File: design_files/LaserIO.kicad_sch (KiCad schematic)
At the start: 25 parts, among them J10 DA15_Receptacle, J11 DB25_Receptacle, U4 74HC245, U5 UA9638CDR, U6 UA9638CDR, U7 74LVC1G3208

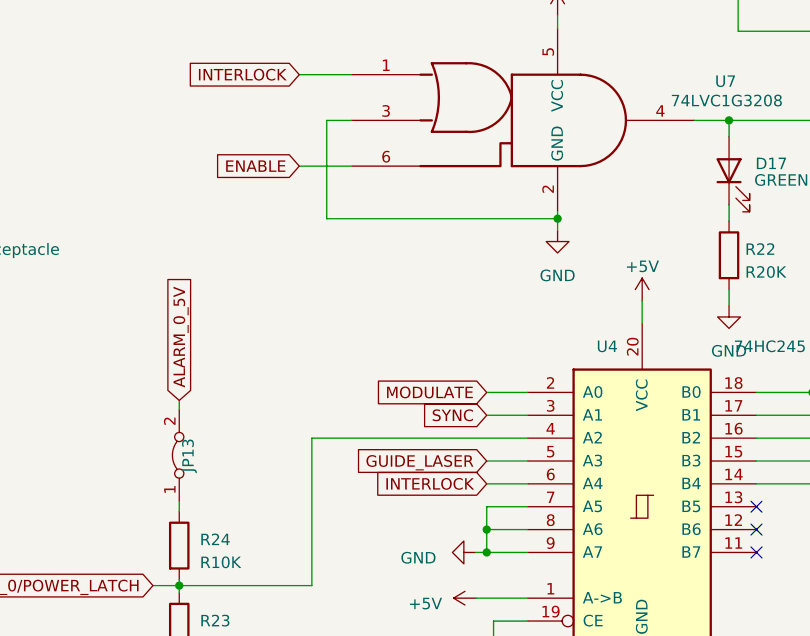
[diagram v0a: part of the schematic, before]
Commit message: Rev 5a
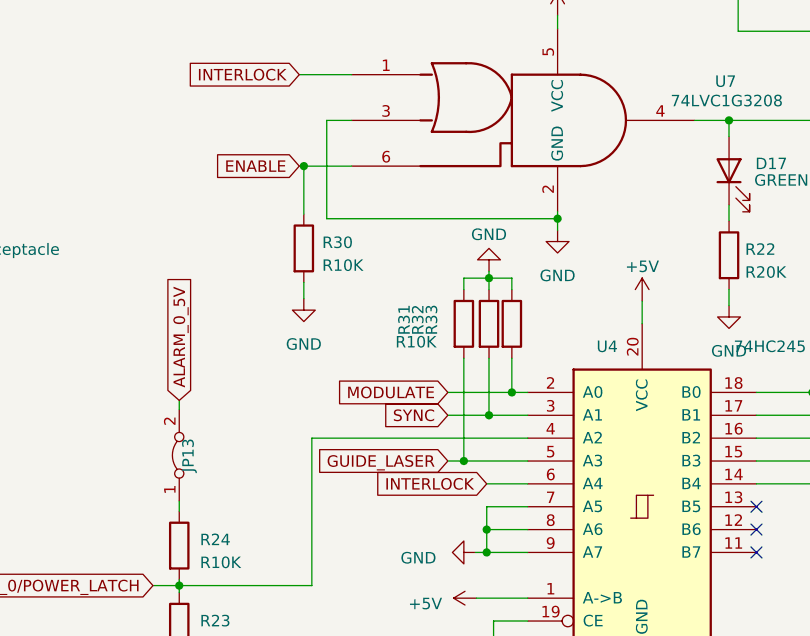
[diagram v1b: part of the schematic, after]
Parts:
- added R30, R31, R32, R33: R10K, LaserBoardR5:R_0603_1608Metric, symbol Device:R
- C10, C7, C8, C9: Notes (none) -> Generic decoupling cap
- R22, R23, R26, R28, R29: MouserPN (none) -> 603-RC0603JR-0720KL; mpn (none) -> RC0603JR-0720KL
- R24, R25, R27: MouserPN (none) -> 603-RC0603JR-0710KL; mpn (none) -> RC0603JR-0710KL
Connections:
- net ENABLE: now also R30.1
- net GND: now also R30.2, R31.1, R32.1, R33.1
- net GUIDE_LASER: now also R31.2
- net MODULATE: now also R33.2
- net SYNC: now also R32.2
